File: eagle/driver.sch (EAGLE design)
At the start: 61 parts, among them IC1 XMEGA128A1, IC10 ST95P08M, IC11 ST95P08M, IC12 ST95P08M, IC13 ST95P08M, IC14 ST95P08M, IC15 ST95P08M, IC16 74AHC1G02DBV, IC17 74AHC1G02DBV, IC18 74AHC1G125DBV, IC19 74AHC1G125DBV, IC2 74AC16244, IC20 ST95P08M, IC21 ST95P08M, IC22 ST95P08M, IC23 ST95P08M, IC24 ST95P08M, IC25 ST95P08M, IC3 74AC16244, IC4 74AC16244, IC5 74AC16244, IC6 74AC16374, IC7 74AC16374, IC8 74AC16374, IC9 74AC16374

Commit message: board layout progress
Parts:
- added C20, C21, C22, C23: 100n, rcl:C-USC0402
- added R11, R12, R13, R14, R15, R16, R17, R18, R19, R20, R21, R22, R23, R24, R25, R26, R27, R28, R29, R30, R31, R32, R33, R34: 33k, rcl:R-US_R0402
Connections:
- net GND: now also C20.2, C21.2, C22.2, C23.2
- net N$29: now also R11.1
- net N$31: now also R12.2
- net N$35: now also R15.1
- net N$41: now also R13.2
- net N$43: now also R16.1
- net N$45: now also R14.2
- net N$47: now also R17.1
- net N$49: now also R18.2
- net N$51: now also R19.1
- net N$53: now also R20.2
- net N$55: now also R21.1
- net N$57: now also R22.2
- net N$64: now also R28.2
- net N$65: now also R27.1
- net N$68: now also R26.2
- net N$70: now also R25.1
- net N$72: now also R24.2
- net N$74: now also R23.1
- net N$76: now also R30.2
- net N$78: now also R29.1
- net N$80: now also R32.2
- net N$82: now also R31.1
- net N$84: now also R34.2
- net N$86: now also R33.1
- net PB7: now also R29.2, R30.1, R31.2, R32.1, R33.2, R34.1
- net PC7: now also R23.2, R24.1, R25.2, R26.1, R27.2, R28.1
- net PH6: now also R17.2, R18.1, R19.2, R20.1, R21.2, R22.1
- net PH7: now also R11.2, R12.1, R13.1, R14.1, R15.2, R16.2
- net VCC: now also C20.1, C21.1, C22.1, C23.1
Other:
- moved on the sheet: IC24, IC25

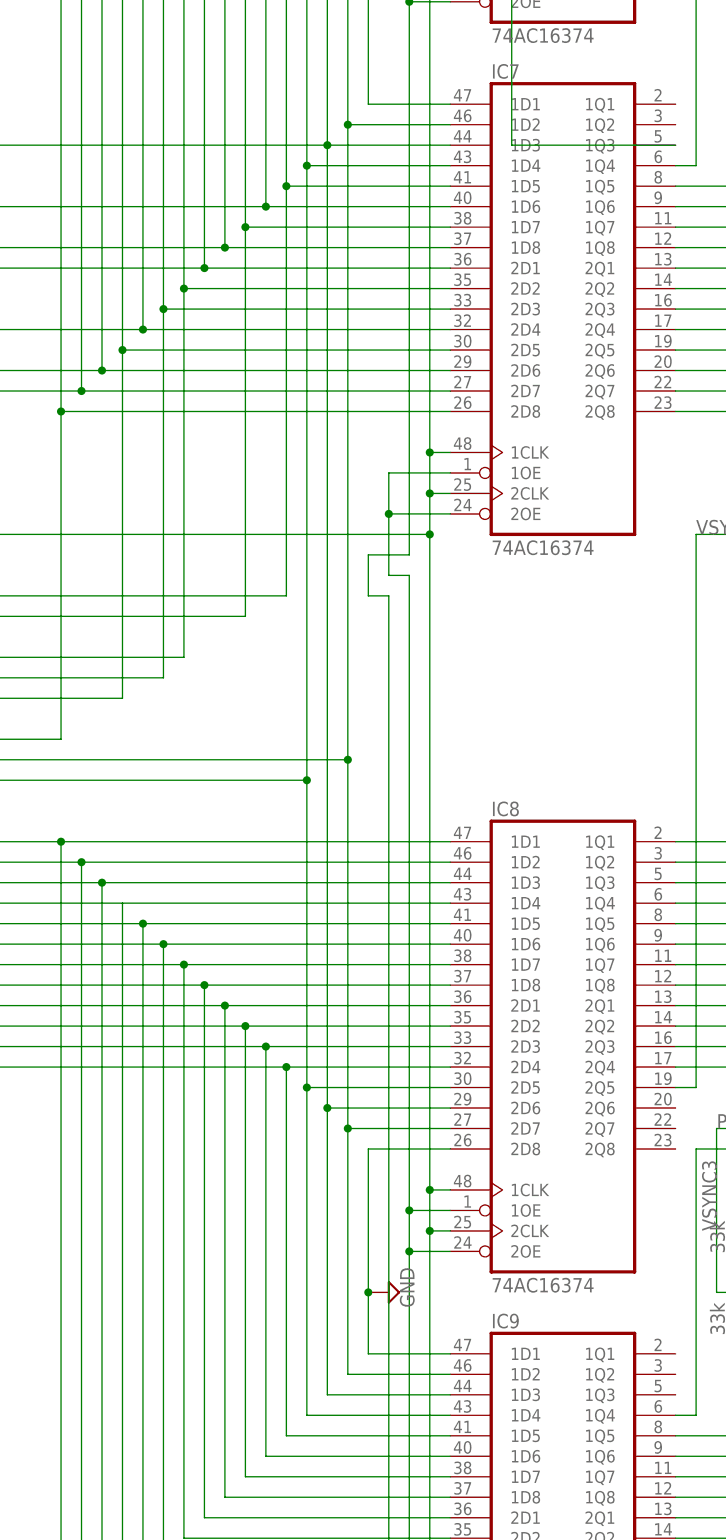
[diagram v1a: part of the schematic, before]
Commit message: finalizing board layout
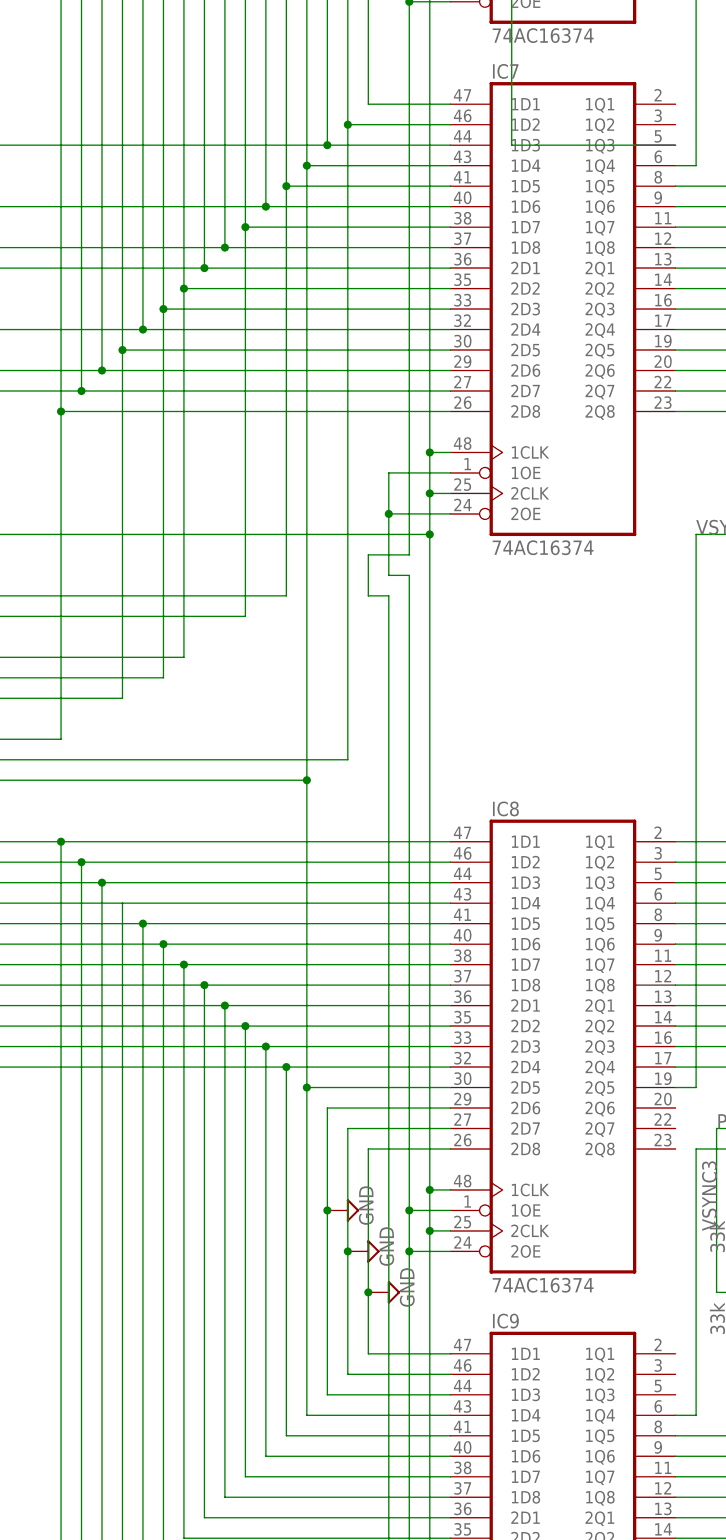
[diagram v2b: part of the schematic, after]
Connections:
- net GND: now also IC8G$1.2D6, IC8G$1.2D7, IC9G$1.1D2, IC9G$1.1D3
- net N$92: no longer IC8G$1.2D7, IC9G$1.1D2
- net N$93: no longer IC8G$1.2D6, IC9G$1.1D3
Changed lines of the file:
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@@
 <part name="R33" library="rcl" library_urn="urn:adsk.eagle:library:334" deviceset="R-US_" device="R0402" package3d_urn="urn:adsk.eagle:package:23547/3" value="33k"/>
 <part name="R34" library="rcl" library_urn="urn:adsk.eagle:library:334" deviceset="R-US_" device="R0402" package3d_urn="urn:adsk.eagle:package:23547/3" value="33k"/>
+<part name="SUPPLY109" library="supply2" library_urn="urn:adsk.eagle:library:372" deviceset="GND" device=""/>
+<part name="SUPPLY110" library="supply2" library_urn="urn:adsk.eagle:library:372" deviceset="GND" device=""/>
 </parts>
 <sheets>
@@
 <attribute name="NAME" x="125.9586" y="222.25" size="1.778" layer="95" rot="R270"/>
 <attribute name="VALUE" x="121.158" y="222.25" size="1.778" layer="96" rot="R270"/>
+</instance>
+<instance part="SUPPLY109" gate="GND" x="78.74" y="228.6" smashed="yes" rot="R90">
+<attribute name="VALUE" x="81.915" y="226.695" size="1.778" layer="96" rot="R90"/>
+</instance>
+<instance part="SUPPLY110" gate="GND" x="76.2" y="233.68" smashed="yes" rot="R90">
+<attribute name="VALUE" x="79.375" y="231.775" size="1.778" layer="96" rot="R90"/>
 </instance>
 </instances>
@@
 <pinref part="C23" gate="G$1" pin="2"/>
 <pinref part="SUPPLY108" gate="GND" pin="GND"/>
+</segment>
+<segment>
+<pinref part="IC9" gate="G$1" pin="1D2"/>
+<pinref part="IC8" gate="G$1" pin="2D7"/>
+<wire x1="88.9" y1="243.84" x2="76.2" y2="243.84" width="0.1524" layer="91"/>
+<wire x1="76.2" y1="243.84" x2="76.2" y2="228.6" width="0.1524" layer="91"/>
+<wire x1="76.2" y1="228.6" x2="76.2" y2="213.36" width="0.1524" layer="91"/>
+<wire x1="76.2" y1="213.36" x2="88.9" y2="213.36" width="0.1524" layer="91"/>
+<pinref part="SUPPLY109" gate="GND" pin="GND"/>
+<junction x="76.2" y="228.6"/>
+</segment>
+<segment>
+<pinref part="IC9" gate="G$1" pin="1D3"/>
+<pinref part="IC8" gate="G$1" pin="2D6"/>
+<wire x1="88.9" y1="246.38" x2="73.66" y2="246.38" width="0.1524" layer="91"/>
+<wire x1="73.66" y1="246.38" x2="73.66" y2="233.68" width="0.1524" layer="91"/>
+<wire x1="73.66" y1="233.68" x2="73.66" y2="210.82" width="0.1524" layer="91"/>
+<wire x1="73.66" y1="210.82" x2="88.9" y2="210.82" width="0.1524" layer="91"/>
+<pinref part="SUPPLY110" gate="GND" pin="GND"/>
+<junction x="73.66" y="233.68"/>
 </segment>
 </net>
@@
 <wire x1="76.2" y1="289.56" x2="76.2" y2="368.3" width="0.1524" layer="91"/>
 <junction x="76.2" y="368.3"/>
-<pinref part="IC8" gate="G$1" pin="2D7"/>
-<wire x1="88.9" y1="243.84" x2="76.2" y2="243.84" width="0.1524" layer="91"/>
-<wire x1="76.2" y1="243.84" x2="76.2" y2="213.36" width="0.1524" layer="91"/>
-<pinref part="IC9" gate="G$1" pin="1D2"/>
-<wire x1="76.2" y1="213.36" x2="88.9" y2="213.36" width="0.1524" layer="91"/>
-<wire x1="76.2" y1="289.56" x2="76.2" y2="243.84" width="0.1524" layer="91"/>
-<junction x="76.2" y="289.56"/>
-<junction x="76.2" y="243.84"/>
 </segment>
 </net>
@@
 <wire x1="-27.94" y1="365.76" x2="73.66" y2="365.76" width="0.1524" layer="91"/>
 <junction x="73.66" y="365.76"/>
-<pinref part="IC8" gate="G$1" pin="2D6"/>
-<wire x1="88.9" y1="246.38" x2="73.66" y2="246.38" width="0.1524" layer="91"/>
-<wire x1="73.66" y1="246.38" x2="73.66" y2="210.82" width="0.1524" layer="91"/>
-<pinref part="IC9" gate="G$1" pin="1D3"/>
-<wire x1="73.66" y1="210.82" x2="88.9" y2="210.82" width="0.1524" layer="91"/>
-<wire x1="73.66" y1="365.76" x2="73.66" y2="246.38" width="0.1524" layer="91"/>
-<junction x="73.66" y="246.38"/>
-</segment>
-</net>
+</segment>
+</net>
